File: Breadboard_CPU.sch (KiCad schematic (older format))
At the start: 20 parts, among them Q5 Q_NPN_CBE, SW3 RESET

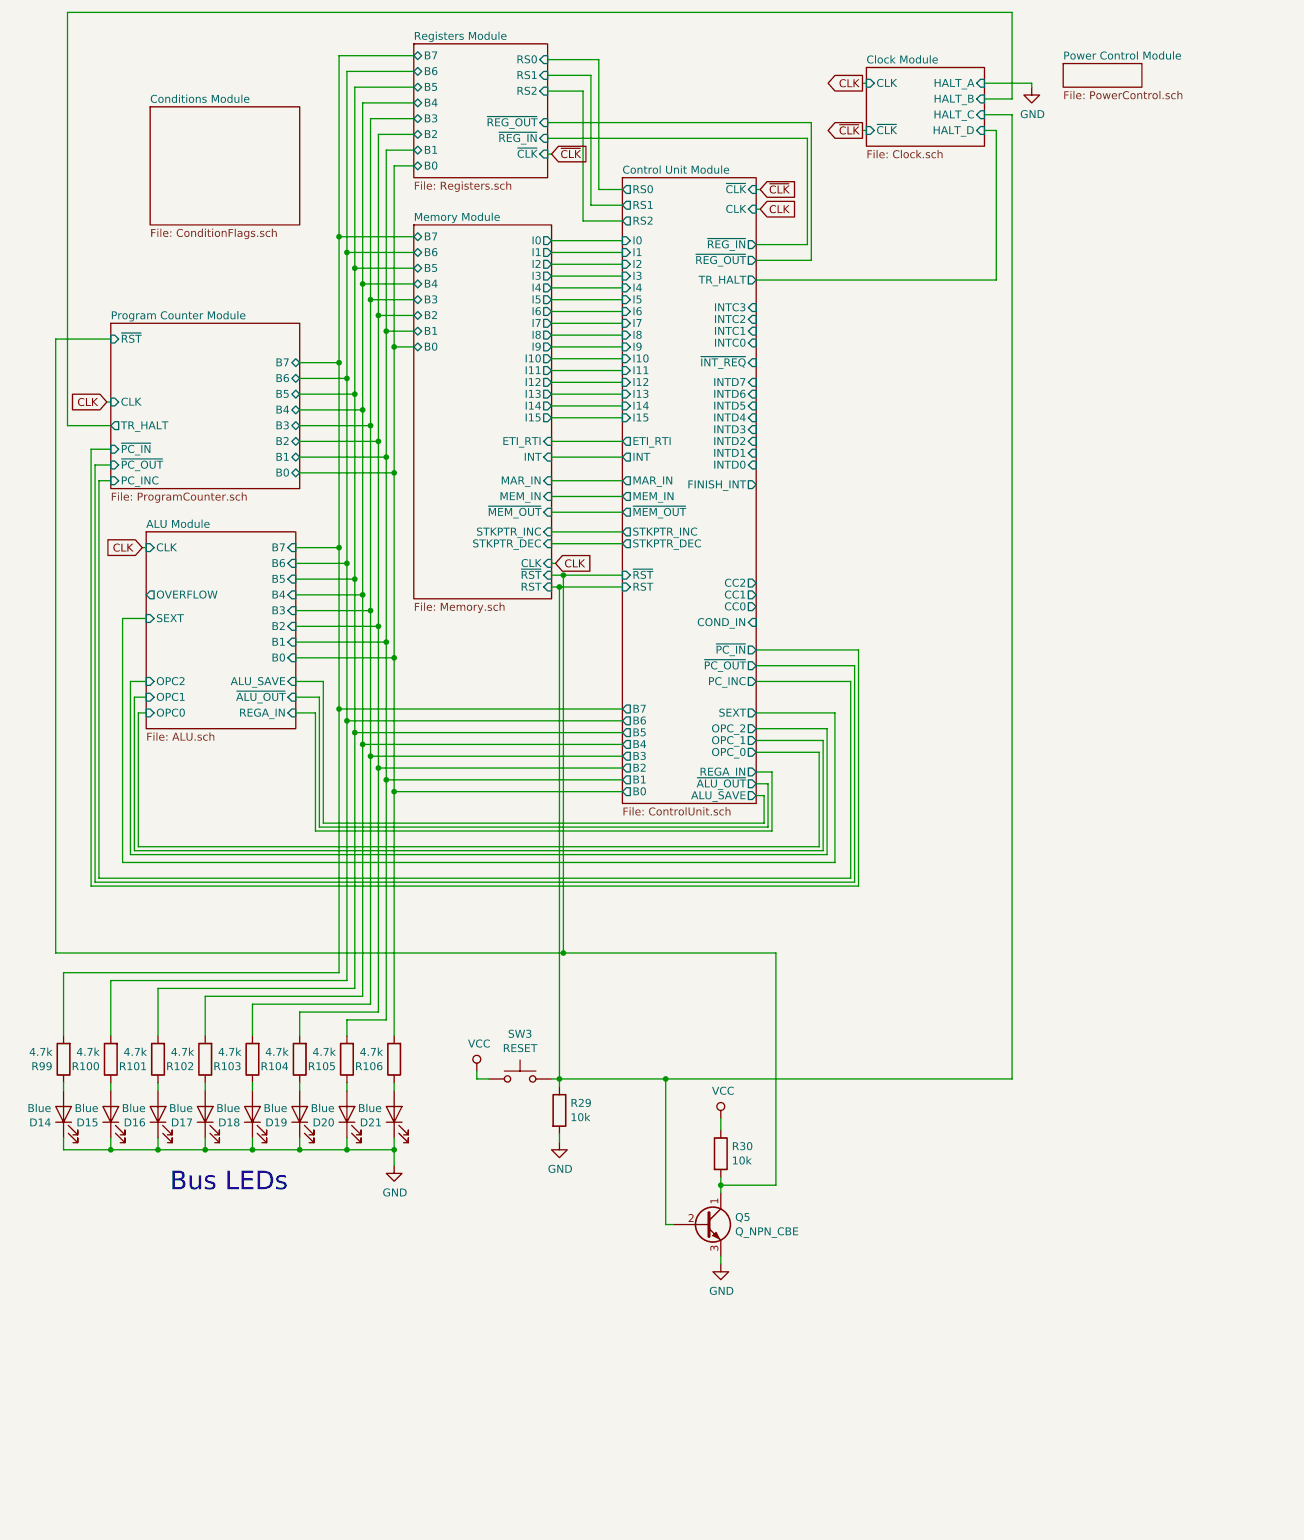
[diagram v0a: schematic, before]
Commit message: Pre non-interrupt split
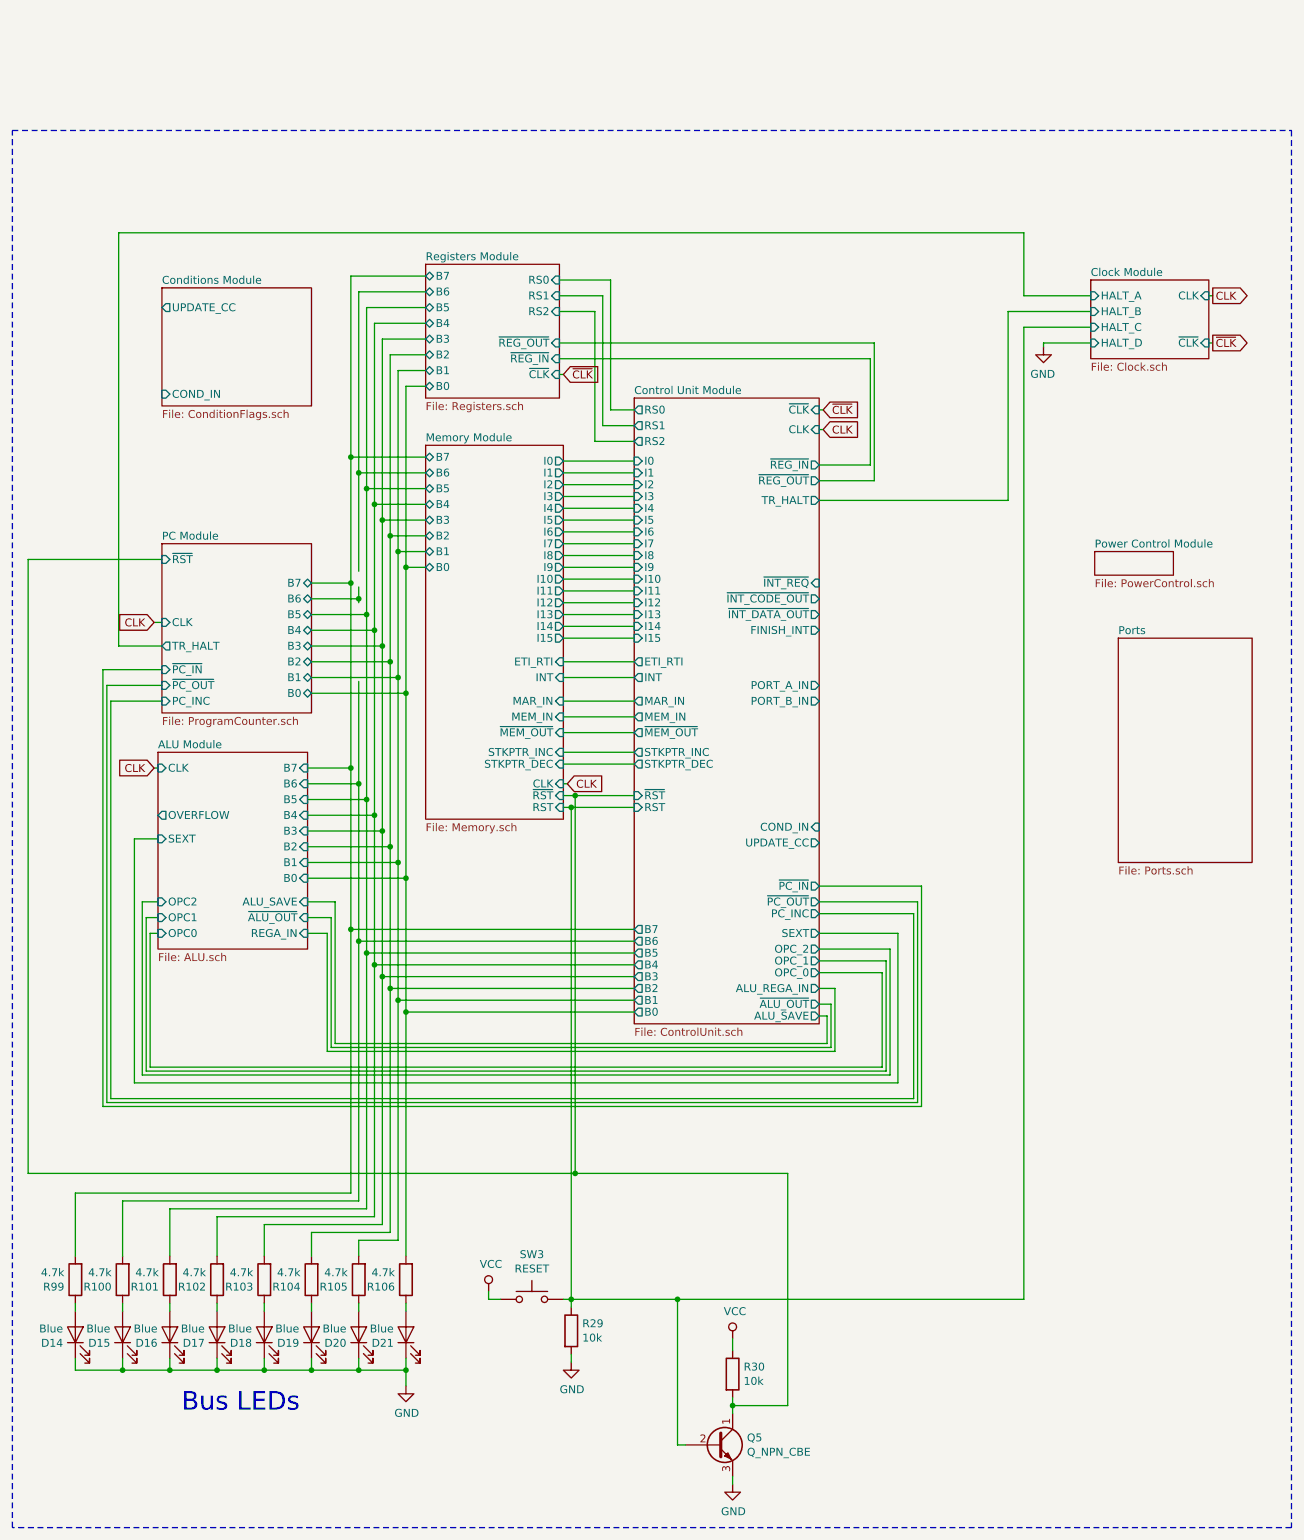
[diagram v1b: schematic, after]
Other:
- moved on the sheet: D14, D15, D16, D17, D18, D19, D20, D21, Q5, R100, R101, R102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
